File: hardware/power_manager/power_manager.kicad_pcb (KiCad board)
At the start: 2 copper layers, 78 x 41.5 mm, 25 parts, among them J1 Conn_01x02_Pin, J2 Conn_01x03_Pin, J3 Conn_01x02_Pin, J4 USB_C_Receptacle_PowerOnly_6P, Q3 AO3401A, U1 TP4054-SOT25R, U2 AP2112K-3.3

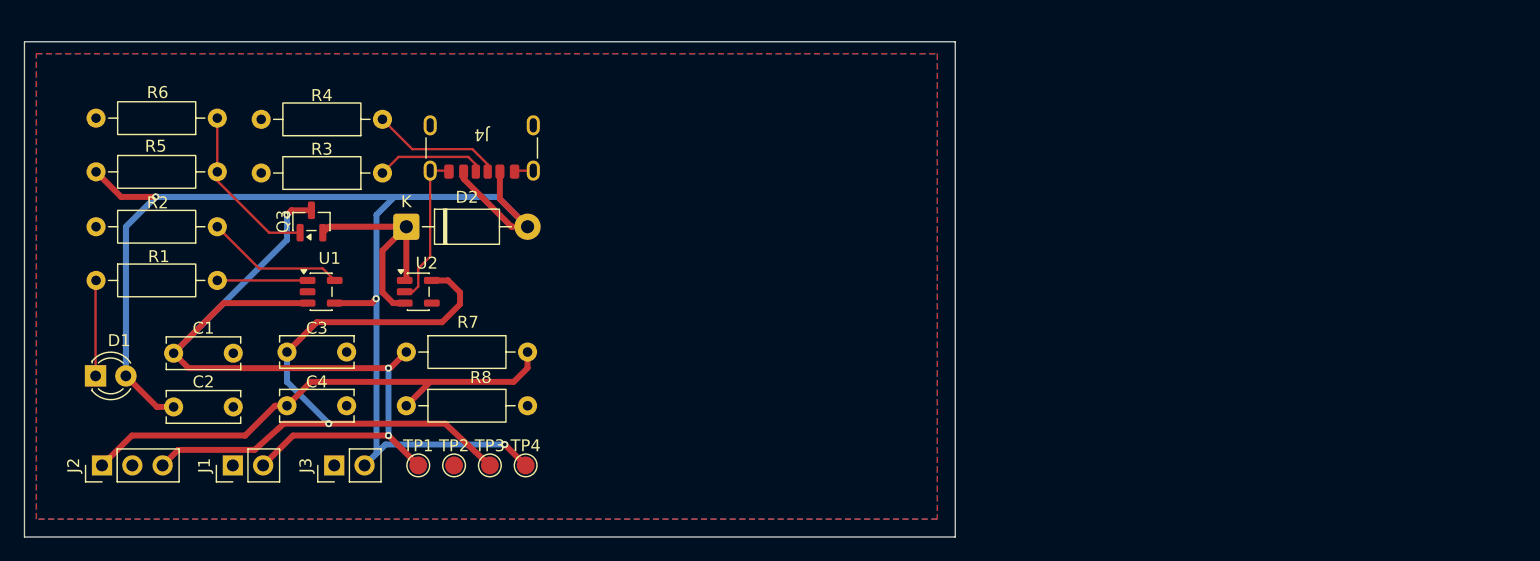
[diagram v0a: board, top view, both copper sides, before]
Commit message: Add: PCB
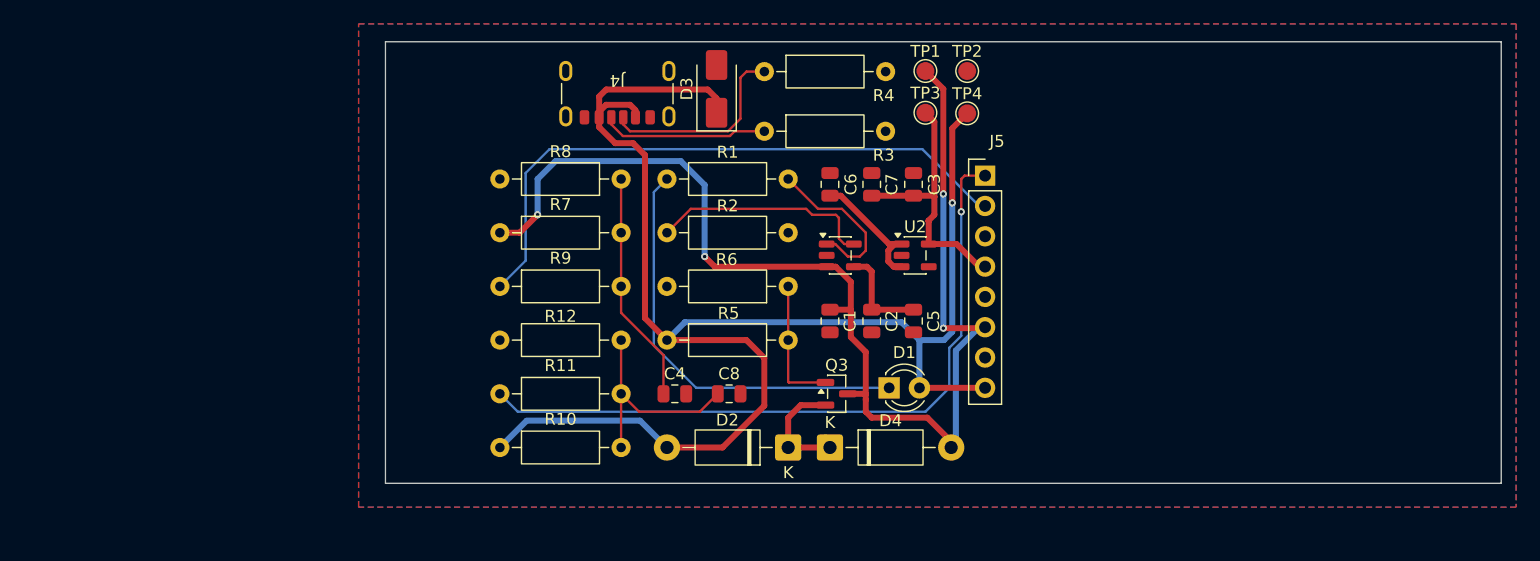
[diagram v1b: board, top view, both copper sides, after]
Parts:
- removed J1, J3: Conn_01x02_Pin, Connector_PinHeader_2.54mm:PinHeader_1x02_P2.54mm_Vertical
- removed J2: Conn_01x03_Pin, Connector_PinHeader_2.54mm:PinHeader_1x03_P2.54mm_Vertical
- added C5: 100nF, Capacitor_SMD:C_0805_2012Metric, F.Cu at (96.0, 58.4)
- added C6: 10uF, Capacitor_SMD:C_0805_2012Metric, F.Cu at (89.0, 47.0)
- added C7: 100nF, Capacitor_SMD:C_0805_2012Metric, F.Cu at (92.5, 47.0)
- added C8: 100nF, Capacitor_SMD:C_0805_2012Metric, F.Cu at (80.5, 64.5)
- added D3: SMAJ5.0A, Diode_SMD:D_SMA, F.Cu at (79.5, 39.0)
- added D4: 1N5819, Diode_THT:D_DO-41_SOD81_P10.16mm_Horizontal, F.Cu at (89.0, 69.0)
- added J5: Conn_01x08_Pin, Connector_PinHeader_2.54mm:PinHeader_1x08_P2.54mm_Vertical, F.Cu at (102.0, 46.2)
- added R10: 200k, Resistor_THT:R_Axial_DIN0207_L6.3mm_D2.5mm_P10.16mm_Horizontal, F.Cu at (61.3, 69.0)
- added R11: 1k, Resistor_THT:R_Axial_DIN0207_L6.3mm_D2.5mm_P10.16mm_Horizontal, F.Cu at (61.3, 64.5)
- added R12: 300k, Resistor_THT:R_Axial_DIN0207_L6.3mm_D2.5mm_P10.16mm_Horizontal, F.Cu at (71.5, 60.0)
- added R9: 1k, Resistor_THT:R_Axial_DIN0207_L6.3mm_D2.5mm_P10.16mm_Horizontal, F.Cu at (61.3, 55.5)
- C1, C2, C4: footprint Capacitor_THT:C_Disc_D6.0mm_W2.5mm_P5.00mm -> Capacitor_SMD:C_0805_2012Metric
- C3: value 10uF -> 1uF; footprint Capacitor_THT:C_Disc_D6.0mm_W2.5mm_P5.00mm -> Capacitor_SMD:C_0805_2012Metric
- R7, R8: value 100k -> 470k
- moved D1 66.5 mm to (94.0, 64.0)
- moved C2 58.9 mm to (92.5, 58.4), turned to -90 degrees
- moved C1 55.1 mm to (89.0, 58.4), turned to -90 degrees
- moved C3 54.3 mm to (96.0, 47.0), turned to 90 degrees
- moved TP2 54.2 mm to (100.5, 37.5)
- moved TP1 53.8 mm to (97.0, 37.5)
- moved R5 49.9 mm to (75.3, 60.0)
- moved R6 49.9 mm to (85.5, 55.5)
- moved R1 48.6 mm to (75.3, 46.5)
- moved TP4 47.3 mm to (100.5, 41.0)
- moved TP3 47.0 mm to (97.0, 41.0)
- moved Q3 46.3 mm to (89.6, 64.5), turned to 0 degrees
- moved U1 43.6 mm to (89.9, 52.9)
- moved U2 41.7 mm to (96.1, 52.9)
- moved R2 37.7 mm to (75.3, 51.0), turned to 0 degrees
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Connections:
- net /BAT_ADC renamed Net-(C4-Pad1)
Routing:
- net /PLUGIN: track 0.00 -> 59.1 mm, vias 0 -> 1
- net /BAT_ADC: track 0.00 -> 51.7 mm
- net /3V3: track 57.6 -> 22.3 mm, vias 1 -> 0
- net /VBAT: track 72.0 -> 102.0 mm, vias 3 -> 4
- net /VIN: track 113.5 -> 142.1 mm, vias 3 -> 1
- net Net-(D1-K): track 8.02 -> 35.6 mm
- net Net-(C4-Pad1): track 43.2 -> 19.5 mm
- net Net-(C8-Pad1): track 0.00 -> 18.3 mm
- net GND: track 14.6 -> 0.00 mm
- net Net-(U1-PROG): track 11.7 -> 18.7 mm
- net Net-(U1-~{CHRG}): track 7.57 -> 13.8 mm
- net Net-(J4-CC1): track 11.0 -> 16.8 mm
- net Net-(J4-CC2): track 9.24 -> 14.0 mm
- net Net-(Q3-G): track 14.1 -> 11.6 mm
- net /VCC: track 20.3 -> 21.8 mm
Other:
- board size 78 x 41.5 mm -> 93.5 x 37 mm
